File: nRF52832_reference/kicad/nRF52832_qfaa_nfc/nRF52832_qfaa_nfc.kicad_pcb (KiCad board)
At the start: 2 copper layers, 40 x 40 mm, 21 parts, among them J1 NFC, X1 32MHz, X2 32.768kHz

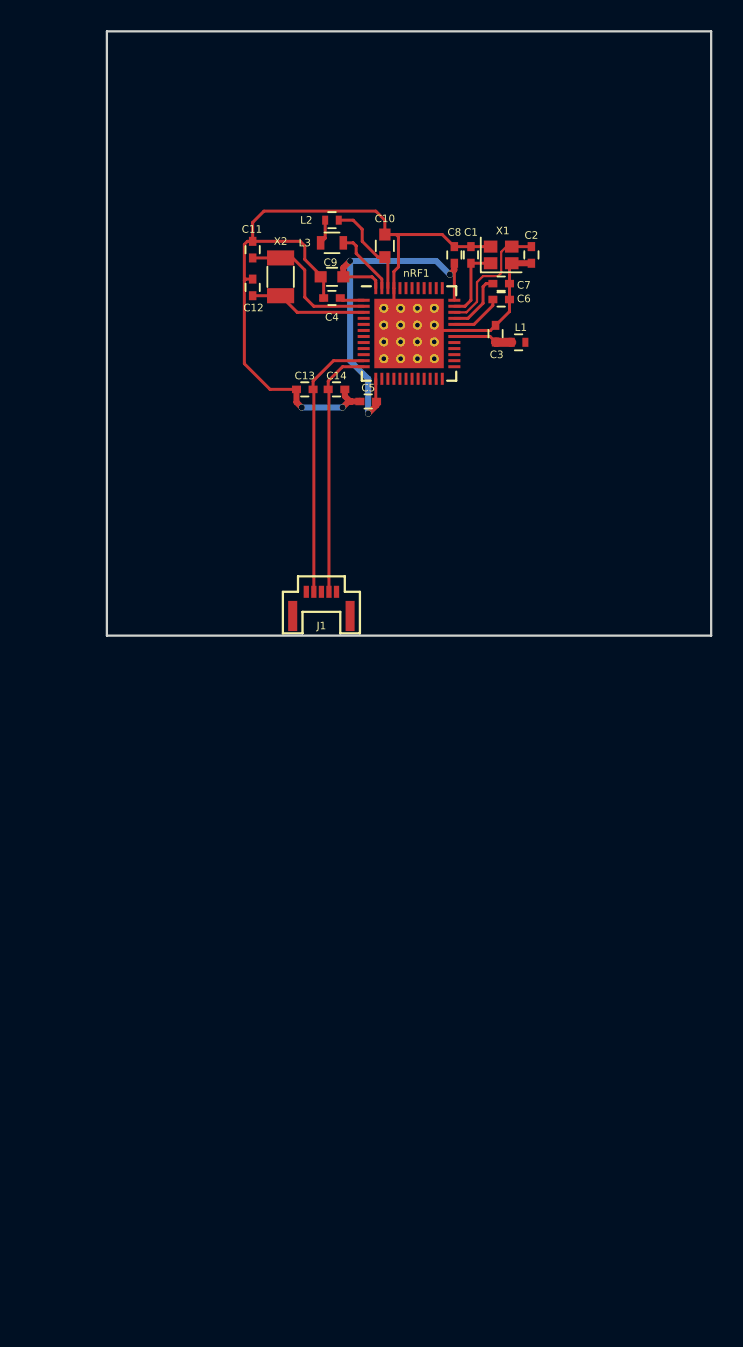
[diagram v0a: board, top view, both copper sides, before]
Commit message: Reference Project nRF52832_qfaa_nfc ready
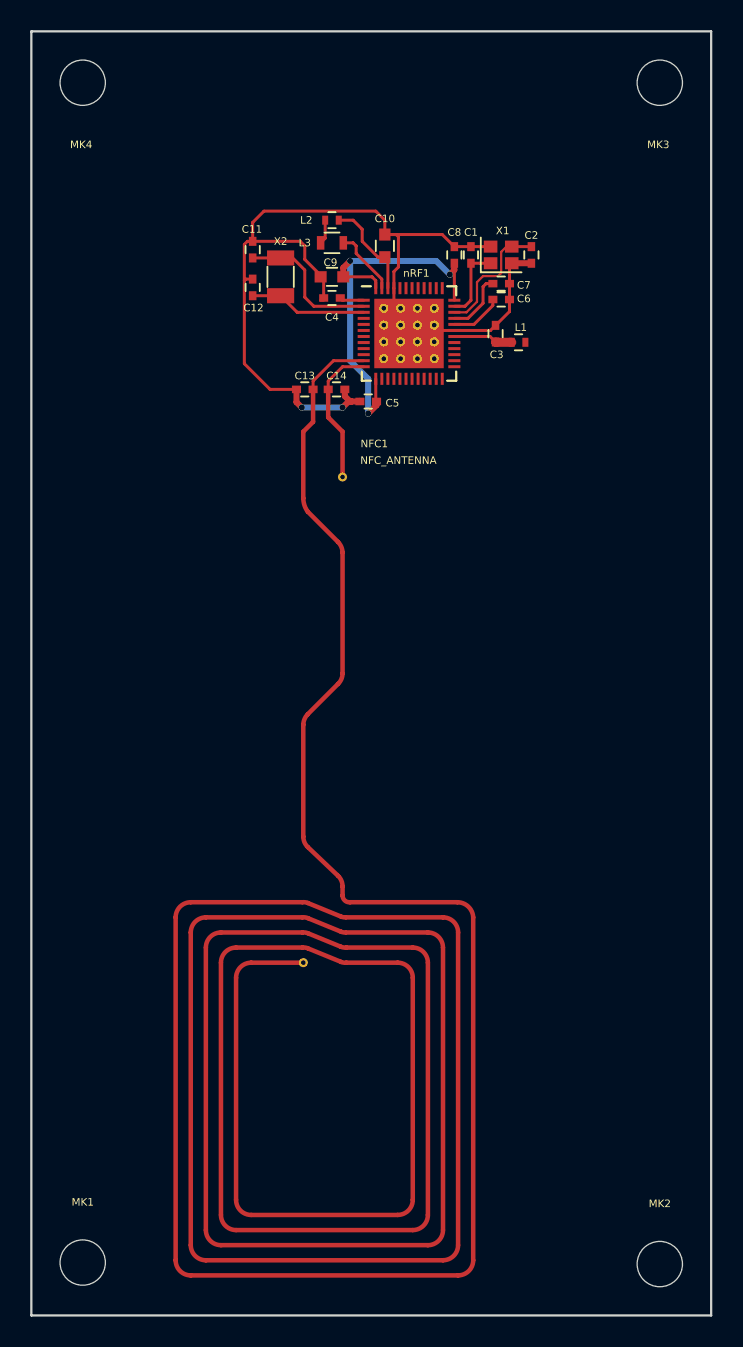
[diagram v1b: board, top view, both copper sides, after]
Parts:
- removed J1: NFC, nRF52:FPC_05P-05mm-RA-SMD_Alt
- added MK1: Mounting_Hole, Nordic_misc:MountingHole_3mm, F.Cu at (78.4, 161.5)
- added MK2: Mounting_Hole, Nordic_misc:MountingHole_3mm, F.Cu at (116.6, 161.6)
- added MK3: Mounting_Hole, Nordic_misc:MountingHole_3mm, F.Cu at (116.6, 83.4)
- added MK4: Mounting_Hole, Nordic_misc:MountingHole_3mm, F.Cu at (78.4, 83.4)
- added NFC1: NFC_ANTENNA, Nordic_misc:Nordic_misc-NFC_ANT, F.Cu at (95.6, 106.5)
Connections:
- L1 pad 2: (no net) -> /RF
- nRF1 pad 10: (no net) -> /P0.08
- nRF1 pad 14: (no net) -> /P0.11
- nRF1 pad 15: (no net) -> /P0.12
- nRF1 pad 16: (no net) -> /P0.13
- nRF1 pad 17: (no net) -> /P0.14
- nRF1 pad 18: (no net) -> /P0.15
- nRF1 pad 19: (no net) -> /P0.16
- nRF1 pad 20: (no net) -> /P0.17
- nRF1 pad 21: (no net) -> /P0.18
- nRF1 pad 22: (no net) -> /P0.19
- nRF1 pad 23: (no net) -> /P0.20
- nRF1 pad 24: (no net) -> /P0.21
- nRF1 pad 25: (no net) -> /SWDCLK
- nRF1 pad 26: (no net) -> /SWDIO
- nRF1 pad 27: (no net) -> /P0.22
- nRF1 pad 28: (no net) -> /P0.23
- nRF1 pad 29: (no net) -> /P0.24
- nRF1 pad 37: (no net) -> /P0.25
- nRF1 pad 38: (no net) -> /P0.26
- nRF1 pad 39: (no net) -> /P0.27
- nRF1 pad 4: (no net) -> /P0.02/AIN0
- nRF1 pad 40: (no net) -> /P0.28/AIN04
- nRF1 pad 41: (no net) -> /P0.29/AIN05
- nRF1 pad 42: (no net) -> /P0.30/AIN06
- nRF1 pad 43: (no net) -> /P0.31/AIN07
- nRF1 pad 44: (no net) -> Net-(nRF1-Pad44)
- nRF1 pad 5: (no net) -> /P0.03/AIN1
- nRF1 pad 6: (no net) -> /P0.04/AIN2
- nRF1 pad 7: (no net) -> /P0.05/AIN3
- nRF1 pad 8: (no net) -> /P0.06
- nRF1 pad 9: (no net) -> /P0.07
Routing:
- net /NFC1: track 18.0 -> 7.67 mm
- net /NFC2: track 16.8 -> 6.63 mm
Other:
- board size 40 x 40 mm -> 45 x 85 mm
